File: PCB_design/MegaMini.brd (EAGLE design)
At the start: 49.2 x 53.3 mm, 25 parts, among them IC1 2560-16AU, IC2 DS1307, J1 AVR_SPI_PROG_3X2NS, Y1 16MHz, Y2 32.768KHz

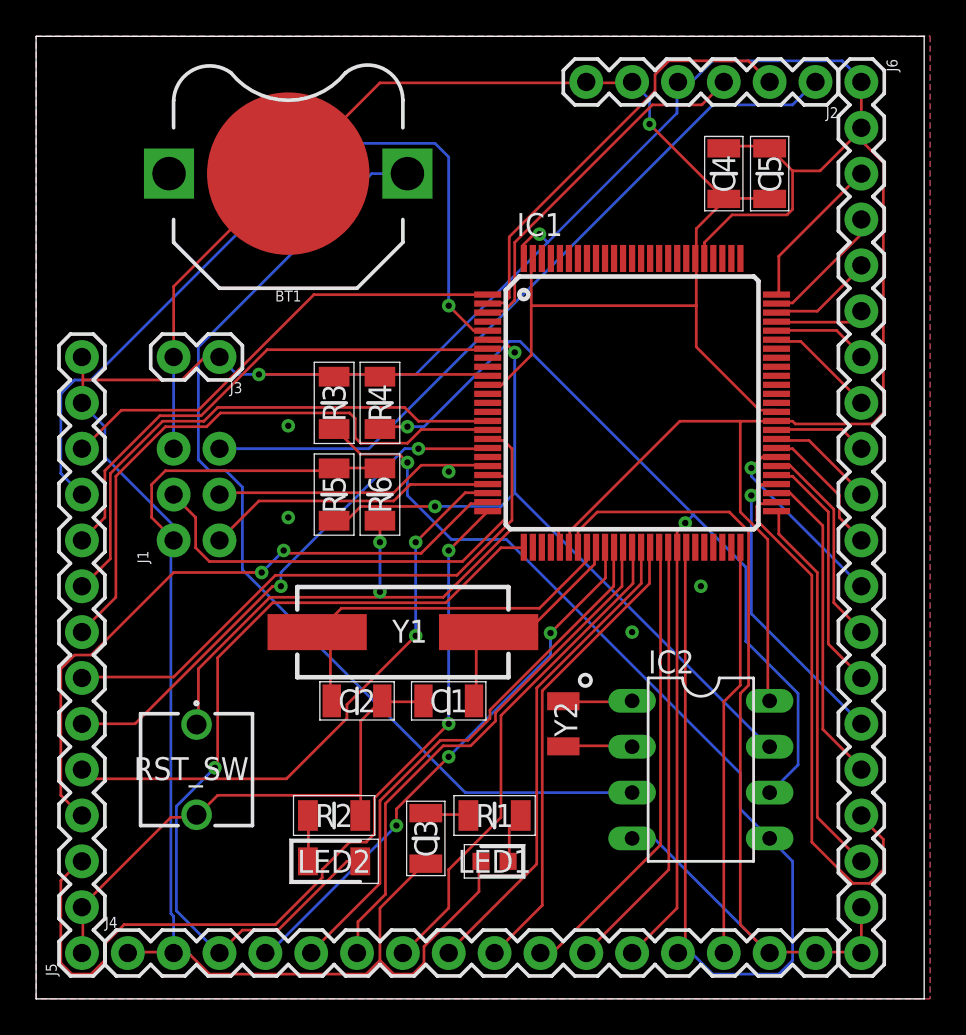
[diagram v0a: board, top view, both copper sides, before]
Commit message: Some little improvements to the pcb
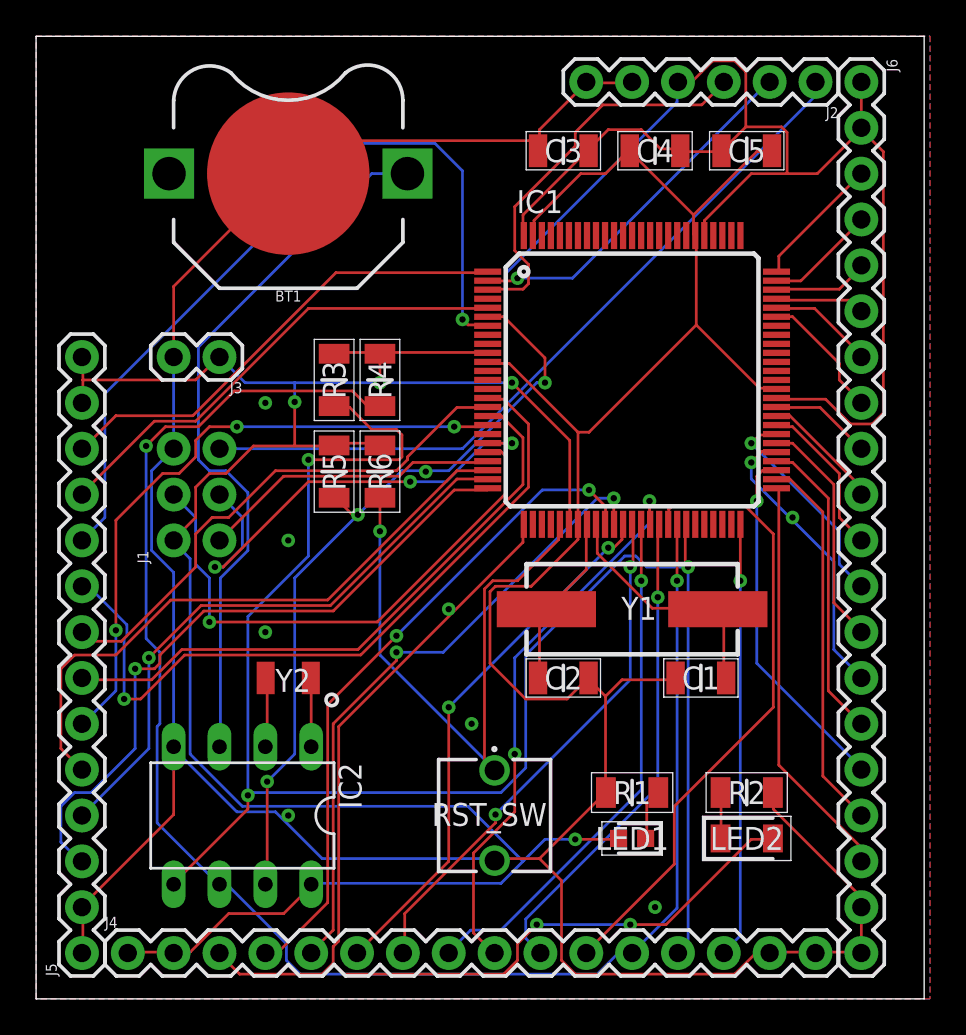
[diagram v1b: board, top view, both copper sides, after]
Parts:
- moved C3 38.9 mm to (29.2, 47.0), turned to 0 degrees
- moved IC2 25.5 mm to (11.4, 10.2), turned to 180 degrees
- moved LED2 22.9 mm to (39.4, 8.89)
- moved R2 22.9 mm to (39.4, 11.4)
- moved RST_SW 16.7 mm to (25.4, 10.2)
- moved Y2 15.5 mm to (14.0, 17.8), turned to 180 degrees
- moved C1 14.0 mm to (36.8, 17.8)
- moved Y1 12.8 mm to (33.0, 21.6)
- moved C2 11.5 mm to (29.2, 17.8)
- moved LED1 7.73 mm to (33.0, 8.89)
- moved R1 7.73 mm to (33.0, 11.4)
- moved C4 4.02 mm to (34.3, 47.0), turned to 0 degrees
- moved C5 1.80 mm to (39.4, 47.0), turned to 180 degrees
- moved R5 1.27 mm to (16.5, 29.2)
- moved R6 1.27 mm to (19.1, 29.2)
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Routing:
- net GND: track 168.5 -> 214.6 mm, vias 6 -> 9
- net PD0: track 67.6 -> 91.5 mm
- net PD1: track 72.9 -> 95.3 mm, vias 1 -> 3
- net PE3: track 44.6 -> 26.8 mm, vias 1 -> 0
- net PB7: track 47.7 -> 64.0 mm, vias 1 -> 2
- net PE5: track 28.4 -> 44.6 mm, vias 0 -> 1
- net N$24: track 56.2 -> 40.0 mm
- net XTAL2: track 21.5 -> 9.64 mm
- net PH3: track 29.7 -> 41.2 mm, vias 0 -> 1
- net VCC: track 226.0 -> 214.9 mm, vias 2 -> 4
- net PB6: track 48.3 -> 37.4 mm, vias 2 -> 1
- net SCK: track 15.6 -> 26.1 mm, vias 0 -> 3
- net PL7: track 24.4 -> 34.8 mm
- net PG1: track 29.8 -> 21.0 mm
- net PL0: track 30.5 -> 37.3 mm, vias 3 -> 2
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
